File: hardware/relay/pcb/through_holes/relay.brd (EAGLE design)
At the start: 51 x 56.2 mm, 12 parts

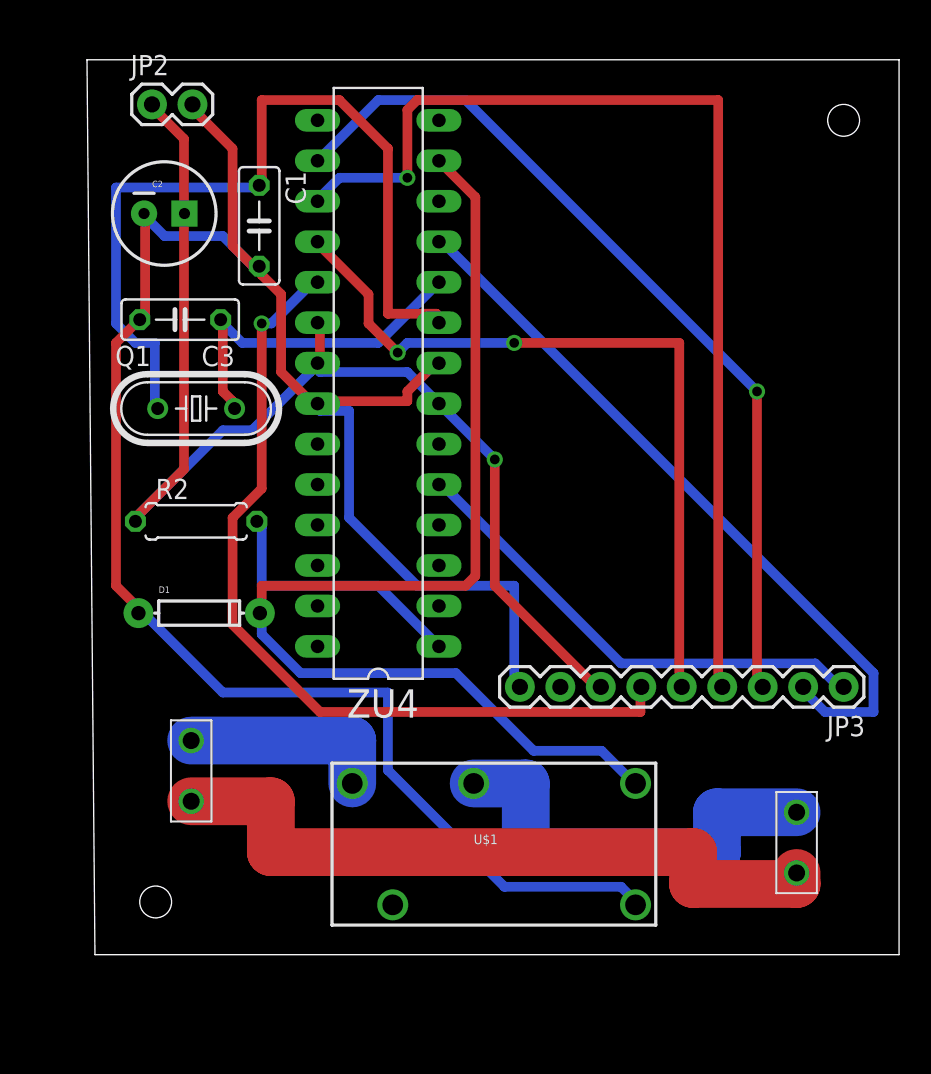
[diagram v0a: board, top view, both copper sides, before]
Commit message: fixes in relay board
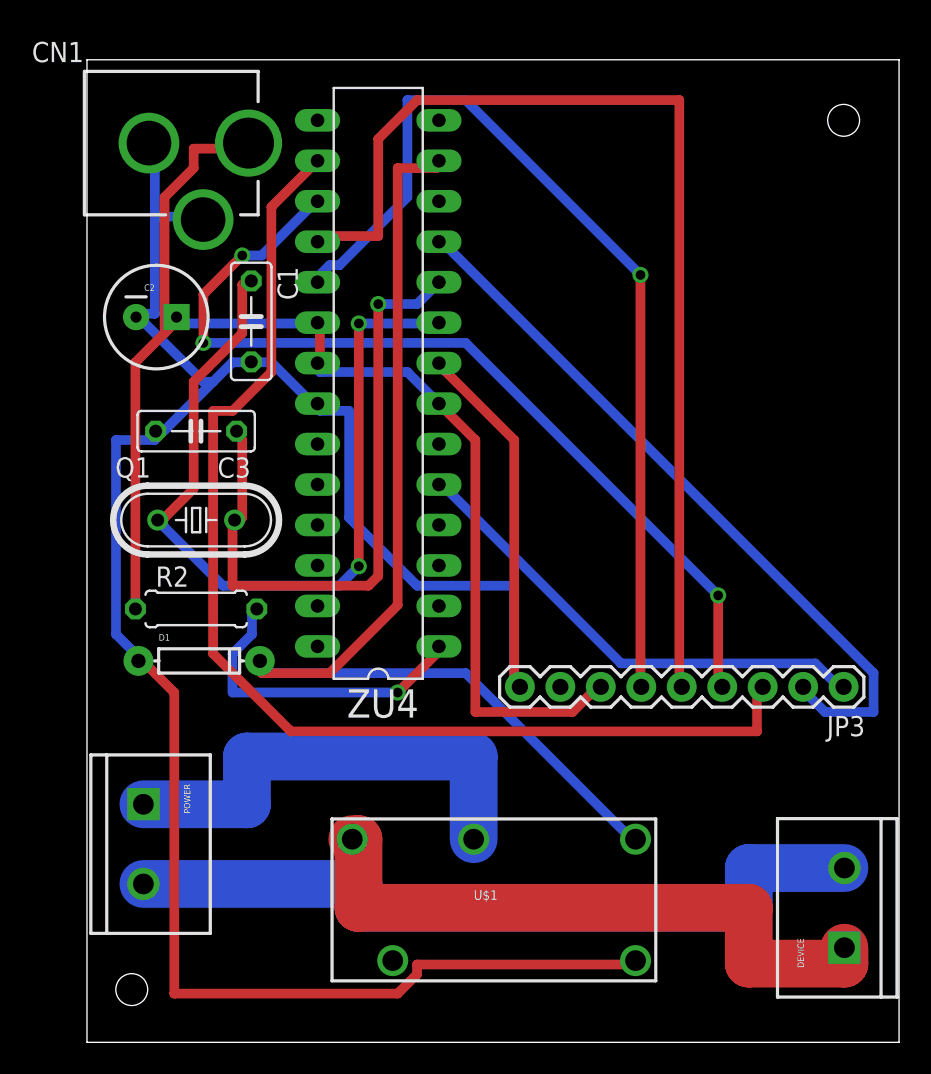
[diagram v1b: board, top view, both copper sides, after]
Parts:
- removed JP2: ARDUINO_POWER, SparkFun-Connectors:1X02
- added CN1: (no value), adafruit:DCJACK_2MM_PTH
- DEVICE, POWER: value M02PTH2 -> M025MM; device SparkFun-Connectors:1X02_BIG -> SparkFun-Connectors:SCREWTERMINAL-5MM-2
- moved DEVICE 43.0 mm to (44.5, 23.0), turned to 90 degrees
- moved POWER 41.0 mm to (0.50, 32.0)
- moved C3 7.07 mm to (3.81, 55.4)
- moved Q1 7.00 mm to (3.81, 49.8)
- moved C2 6.52 mm to (1.31, 62.6)
- moved C1 6.02 mm to (7.27, 62.3)
- moved R2 5.50 mm to (3.81, 44.3)
- moved U$1 3.50 mm to (22.5, 26.0)
- moved D1 3.00 mm to (4.00, 41.0)
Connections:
- net GND: now also CN1.GND, CN1.GNDBREAK; no longer JP2.2
- net N$7: now also POWER.1; no longer POWER.P$1
- net N$8: now also DEVICE.1; no longer DEVICE.P$1
- net N$9: now also DEVICE.2, POWER.2; no longer DEVICE.P$2, POWER.P$2
- net VCC: now also CN1.PWR; no longer JP2.1
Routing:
- net N$8: track 12.8 -> 39.7 mm
- net XTAL2: track 21.8 -> 41.0 mm, vias 0 -> 1
- net GND: track 135.8 -> 154.2 mm
- net N$19: track 48.6 -> 66.9 mm, vias 2 -> 0
- net N$6: track 55.5 -> 73.5 mm, vias 1 -> 0
- net N$20: track 67.2 -> 57.3 mm, vias 1 -> 3
- net VCC: track 77.7 -> 84.7 mm, vias 1 -> 0
- net N$5: track 53.6 -> 59.1 mm
- net N$9: track 43.9 -> 48.0 mm
- net N$3: track 16.8 -> 20.2 mm, vias 0 -> 1
- net N$7: track 27.1 -> 28.9 mm
- net N$26: track 71.1 -> 69.7 mm
- net N$4: track 53.2 -> 52.8 mm, vias 0 -> 2
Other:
- board size 51 x 56.2 mm -> 51 x 61.7 mm
